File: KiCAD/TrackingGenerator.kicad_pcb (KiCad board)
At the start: 4 copper layers, 102.9 x 62.2 mm, 65 parts, among them IC1 ABA-52563-BLKG, IC2 ABA-52563-BLKG, IC3 ABA-52563-BLKG, J1 Conn_Coaxial, J2 Conn_Coaxial, J3 Screw_Terminal_01x02, J4 Conn_Coaxial, M1 PAM-42, U1 L7805

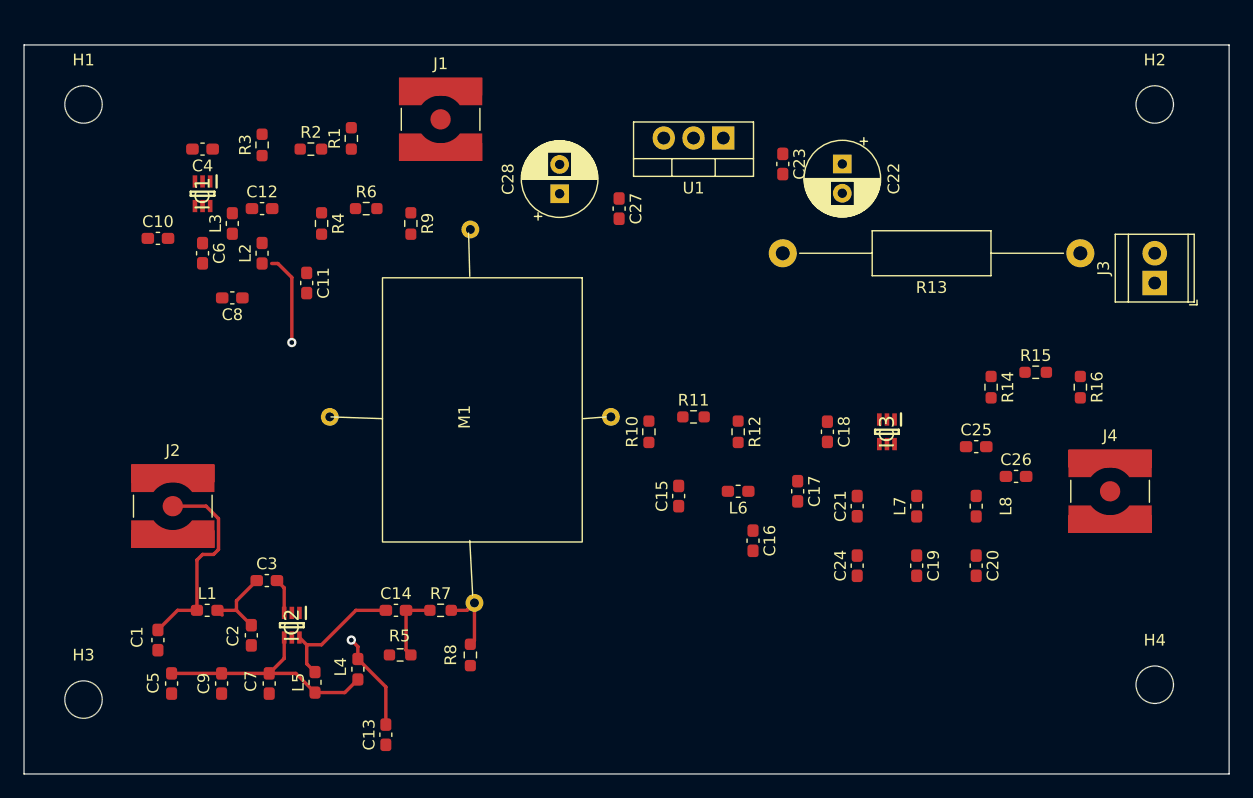
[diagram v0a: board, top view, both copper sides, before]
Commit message: More routing work
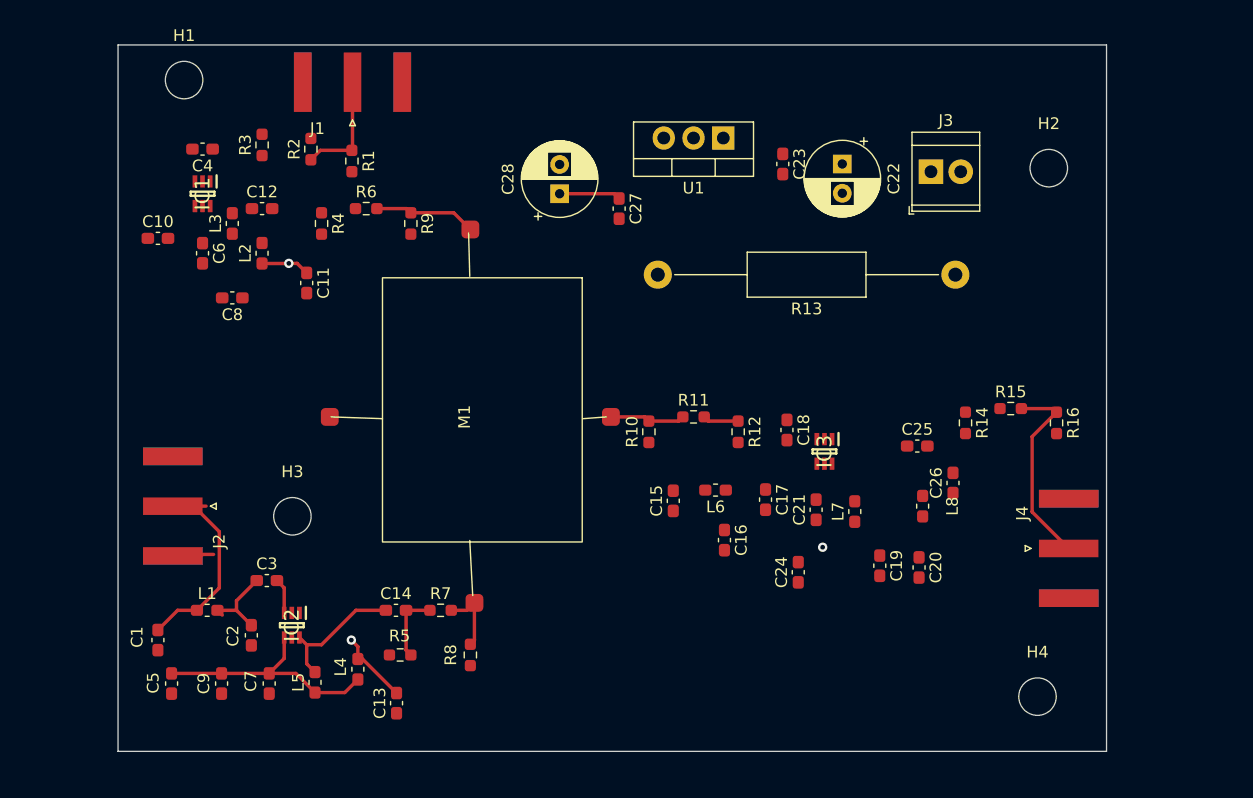
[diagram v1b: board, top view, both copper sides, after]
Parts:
- J1, J2, J4: footprint Connector_Coaxial:SMA_Amphenol_132134-10_Vertical -> Connector_Coaxial:SMA_Amphenol_132289_EdgeMount
- moved H3 23.7 mm to (85.1, 117.7)
- moved J3 21.3 mm to (139.6, 88.3), turned to 0 degrees
- moved R13 10.8 mm to (141.7, 97.1)
- moved H2 10.6 mm to (149.7, 88.0)
- moved H4 10.1 mm to (148.7, 133.1)
- moved H1 8.83 mm to (75.9, 80.5)
- moved J1 8.16 mm to (90.3, 80.6), turned to 90 degrees
- moved J4 6.02 mm to (151.4, 120.4)
- moved IC3 5.59 mm to (130.6, 112.2)
- moved C26 5.41 mm to (141.5, 114.9), turned to 90 degrees
- moved L7 5.30 mm to (133.1, 117.3)
- moved C24 5.06 mm to (128.3, 122.5)
- moved C25 5.03 mm to (138.5, 111.7)
- moved C20 4.88 mm to (138.6, 122.1)
- moved L8 4.57 mm to (138.9, 116.8)
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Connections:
- H1 pad : GNDPWR -> (no net)
- H2 pad : GNDPWR -> (no net)
- H3 pad : GNDPWR -> (no net)
- H4 pad : GNDPWR -> (no net)
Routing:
- net +5V: track 43.7 -> 15.8 mm, vias 1 -> 3
- net Net-(J4-Pad1): track 0.00 -> 16.9 mm
- net Net-(J1-Pad1): track 0.00 -> 9.68 mm
- net Net-(M1-Pad1): track 0.00 -> 8.71 mm
- net Net-(M1-Pad4): track 0.00 -> 6.43 mm
- net Net-(C15-Pad2): track 0.00 -> 3.05 mm
- net Net-(C1-Pad1): track 17.5 -> 19.2 mm
- net GNDPWR: track 0.00 -> 1.62 mm
- net (no net): vias 1 -> 0
- added copper zone on In1.Cu, net +5V
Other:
- board size 102.9 x 62.2 mm -> 84.4 x 60.3 mm
